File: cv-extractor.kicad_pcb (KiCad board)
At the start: 2 copper layers, 30 x 100 mm, 31 parts, among them J1 mono-jack, J2 mono-jack, J3 power_connector_10pos, U1 TL074

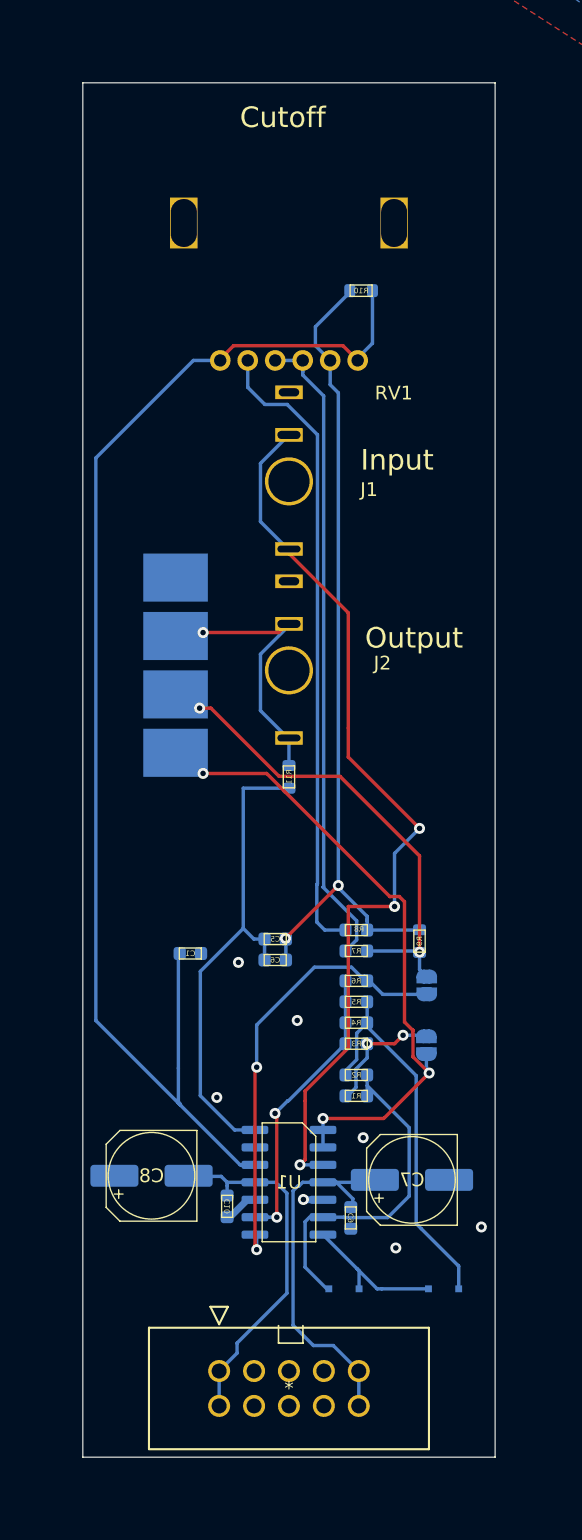
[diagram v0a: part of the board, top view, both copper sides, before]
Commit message: havent been good about commits, its at V4 now
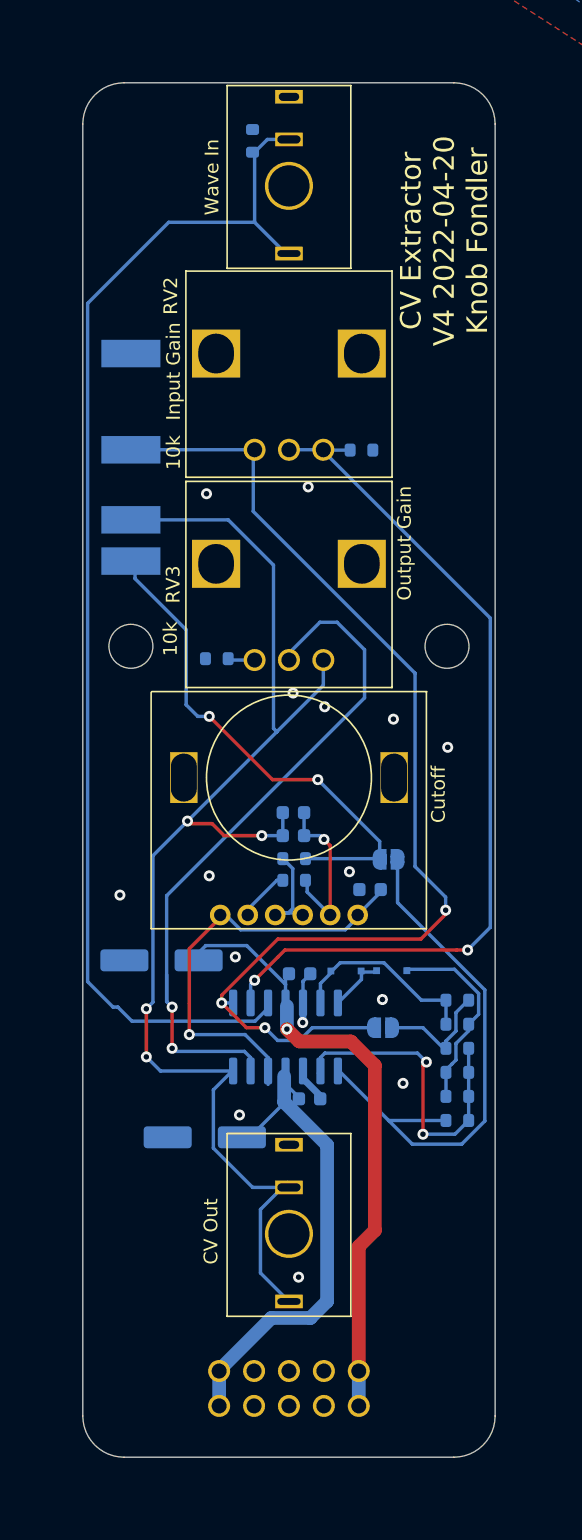
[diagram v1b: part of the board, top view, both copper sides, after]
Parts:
- removed R10: 100k, Resistor_SMD:R_0603_1608Metric
- removed R11: 1k, Resistor_SMD:R_0603_1608Metric
- added H1: Hole, MountingHole:MountingHole_3.2mm_M3, F.Cu at (111.5, 61.0)
- added H2: Hole, MountingHole:MountingHole_3.2mm_M3, F.Cu at (88.5, 61.0)
- added R12: 1k, Resistor_SMD:R_0603_1608Metric, B.Cu at (105.3, 46.7)
- added RD1: 1M, Resistor_SMD:R_0603_1608Metric, B.Cu at (97.3, 24.2)
- added RV2: 10k, matterwave:pot_bourns_PTV09, F.Cu at (100.0, 39.7)
- added RV3: 10k, matterwave:pot_bourns_PTV09, F.Cu at (100.0, 55.0)
- C1, C5, C6: value 10uF -> 470nF
- J1: value mono-jack -> Wave In
- J2: value mono-jack -> CV Out
- R7, R8: value 2.2k -> 1k
- R9: value 100k -> 1k
- TP4: value Abs -> GND
- moved J2 41.0 mm to (100.0, 103.8)
- moved RV1 40.3 mm to (100.0, 80.5)
- moved R9 25.3 mm to (94.8, 61.9), turned to 0 degrees
- moved C7 24.2 mm to (90.7, 83.8), turned to 180 degrees
- moved D2 23.5 mm to (107.5, 84.6)
- moved D1 23.1 mm to (104.2, 84.6)
- moved TP1 22.3 mm to (88.5, 46.7)
- moved J1 21.5 mm to (100.0, 27.5)
- moved C9 18.2 mm to (100.8, 84.8), turned to 180 degrees
- moved TP4 16.6 mm to (88.5, 39.7)
- moved C1 13.9 mm to (105.9, 78.7), turned to 0 degrees
- moved R6 12.5 mm to (112.2, 95.5), turned to 0 degrees
- moved C6 10.8 mm to (100.3, 73.1)
- moved U1 10.6 mm to (99.8, 89.4), turned to 270 degrees
- moved TP2 10.2 mm to (88.5, 54.8)
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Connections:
- J2 pad 2: Net-(J2-Pad2) -> Net-(C5-Pad2)
- J2 pad 3: Net-(J2-Pad2) -> Net-(C5-Pad2)
- R9 pad 1: Net-(C5-Pad1) -> GND
- R9 pad 2: Net-(JP2-Pad2) -> Net-(R9-Pad2)
- TP3 pad 1: Net-(J2-Pad2) -> Net-(C5-Pad2)
- U1 pad 13: Net-(C5-Pad2) -> Net-(RV3-Pad2)
- U1 pad 2: Net-(JP1-Pad1) -> Net-(R12-Pad2)
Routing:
- net Net-(R12-Pad2): track 0.00 -> 65.0 mm, vias 0 -> 2
- net Net-(C1-Pad2): track 96.6 -> 31.8 mm, vias 0 -> 1
- net Net-(C5-Pad2): track 36.9 -> 97.9 mm, vias 0 -> 4
- net Net-(RV3-Pad2): track 0.00 -> 51.8 mm, vias 0 -> 2
- net Net-(C5-Pad1): track 59.9 -> 12.4 mm, vias 2 -> 1
- net Net-(R8-Pad1): track 46.3 -> 3.50 mm
- net Net-(R7-Pad1): track 47.9 -> 6.55 mm
- net Net-(JP1-Pad1): track 44.4 -> 81.2 mm
- net Net-(J1-Pad2): track 66.1 -> 90.3 mm, vias 3 -> 0
- net Net-(J2-Pad2): track 18.1 -> 0.00 mm, vias 1 -> 0
- net +12V: track 29.3 -> 45.6 mm, vias 0 -> 1
- net Net-(D2-Pad2): track 28.1 -> 14.6 mm
- net -12V: track 27.5 -> 40.8 mm
- net Net-(D1-Pad1): track 24.7 -> 14.2 mm
- net Net-(JP2-Pad1): track 32.5 -> 39.7 mm, vias 2 -> 0
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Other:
- outline, holes or cut-outs redrawn
- board text added: "CV Extractor V4 2022-04-20 Knob Fondler"
- board text removed: "-12V"
- board text removed: "CV Extractor V2 2021-10-29 Knob Fondler"
- board text removed: "Cutoff"
- board text removed: "Input"
- board text removed: "Output"
